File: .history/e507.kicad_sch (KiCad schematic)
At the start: 12 parts, among them J1 Micro_SD_Card, SW1 TS-1088-AR02016, SW2 TS-1088-AR02016, U2 ESP32-S3-WROOM-1

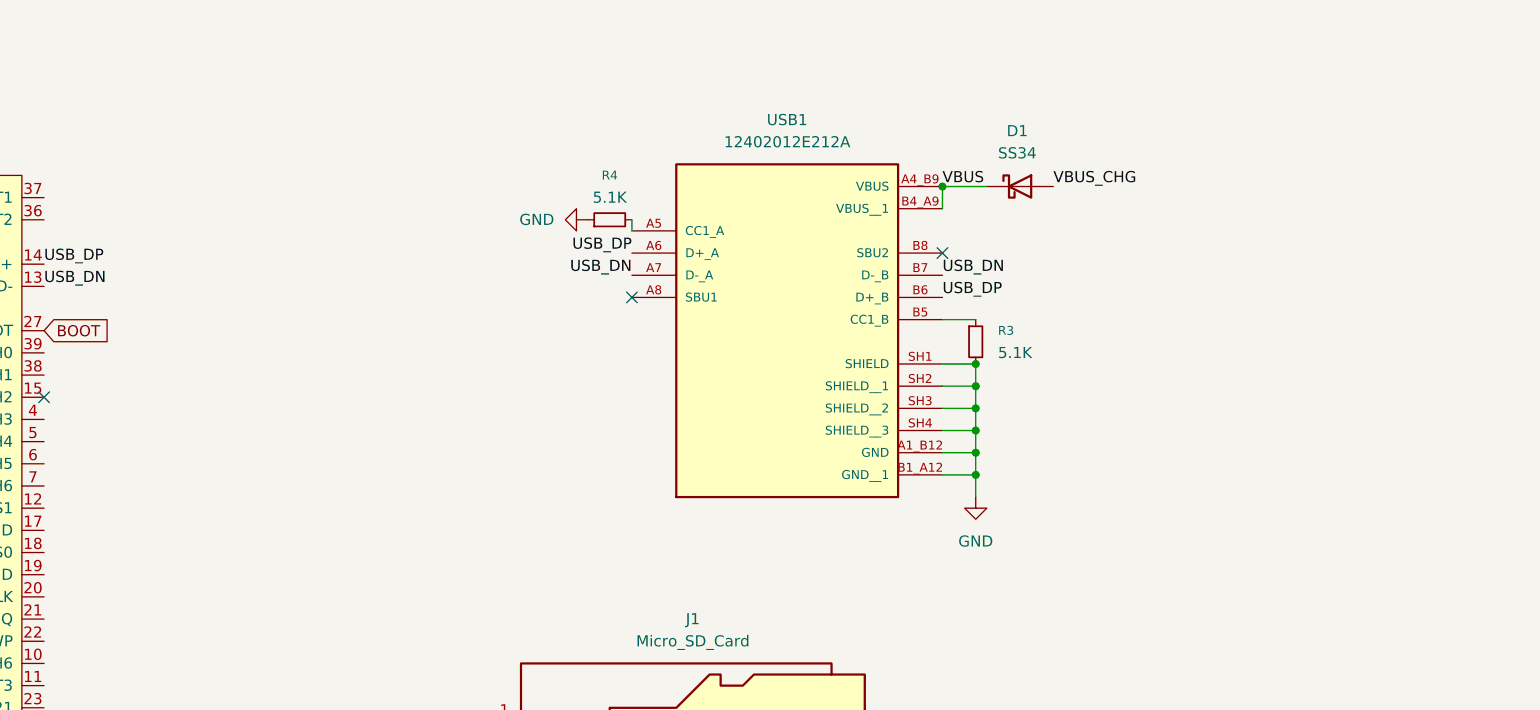
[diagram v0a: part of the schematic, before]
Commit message: download bq25185
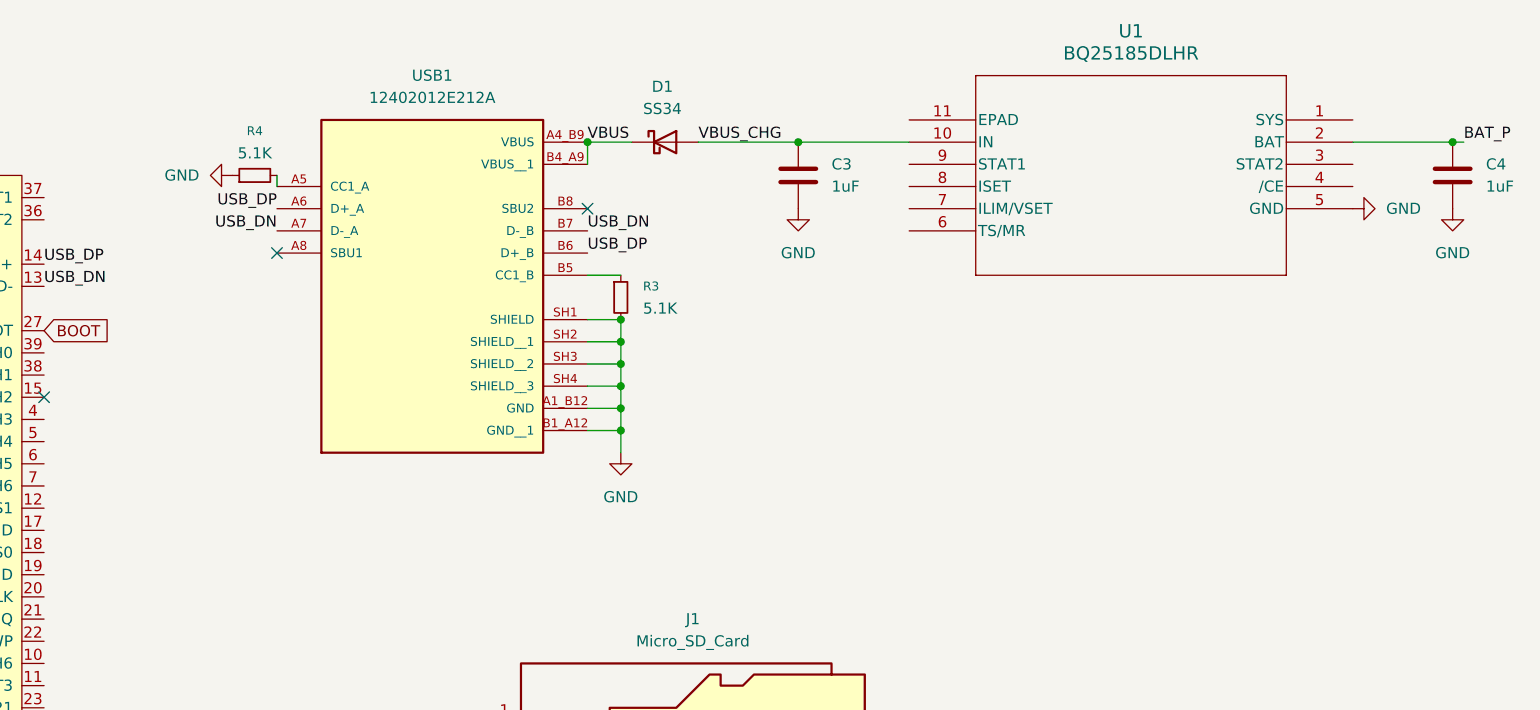
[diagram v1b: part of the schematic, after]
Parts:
- added C3, C4: 1uF, Package_SON:WSON-6-1EP_3x3mm_P0.95mm, symbol Device:C
- added U1: BQ25185DLHR, WSON10_DLH_TEX, symbol bq25185:BQ25185DLHR
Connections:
- net GND: now also C3.1, C4.1, U1.5 (GND)
- net VBUS_CHG: now also C3.2, U1.10 (IN)
- new net BAT_P: C4.2, U1.2 (BAT)
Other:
- moved on the sheet: D1, R3, R4, USB1
